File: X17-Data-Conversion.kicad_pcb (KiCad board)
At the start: 2 copper layers, 41.5 x 30.7 mm, 28 parts, among them J1 Conn_01x05, J4 Conn_01x12_Pin, U2 STM32F091CCTx, U3 MAX485E, U4 MAX7375AXR805+T, U5 AZ1117IH-3.3TRG1

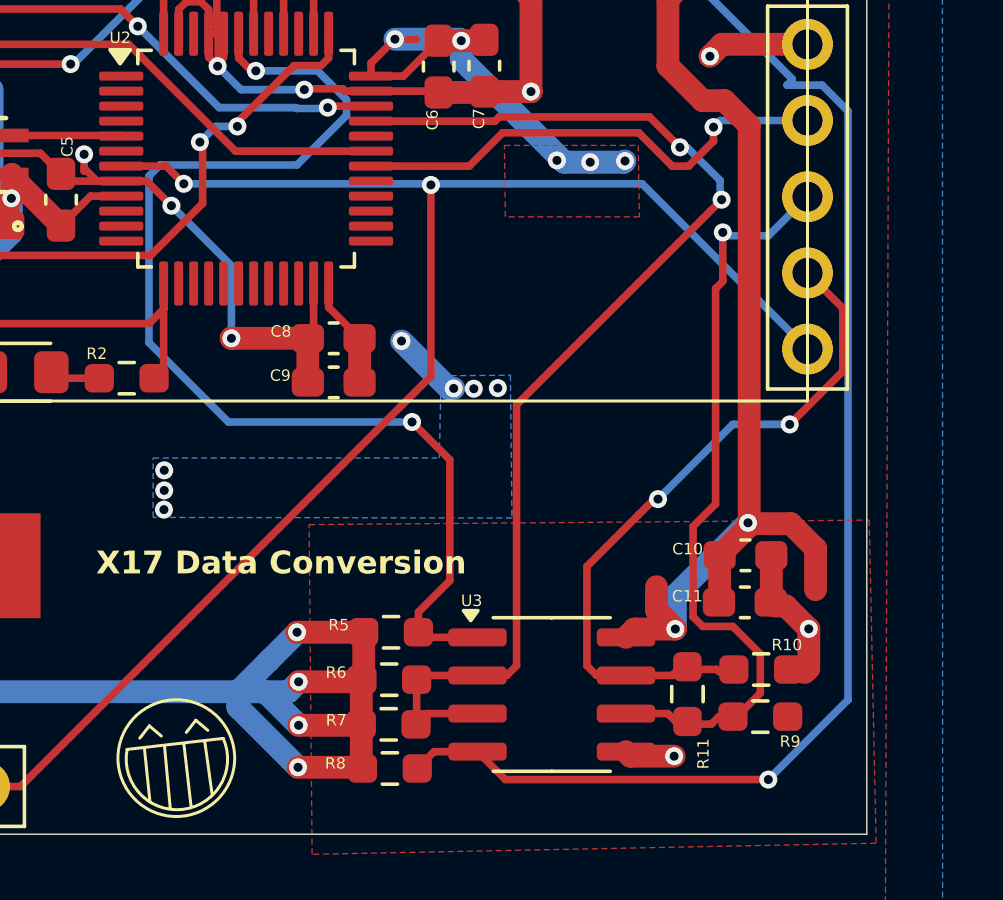
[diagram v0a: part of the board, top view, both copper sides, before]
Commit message: daniel lookie
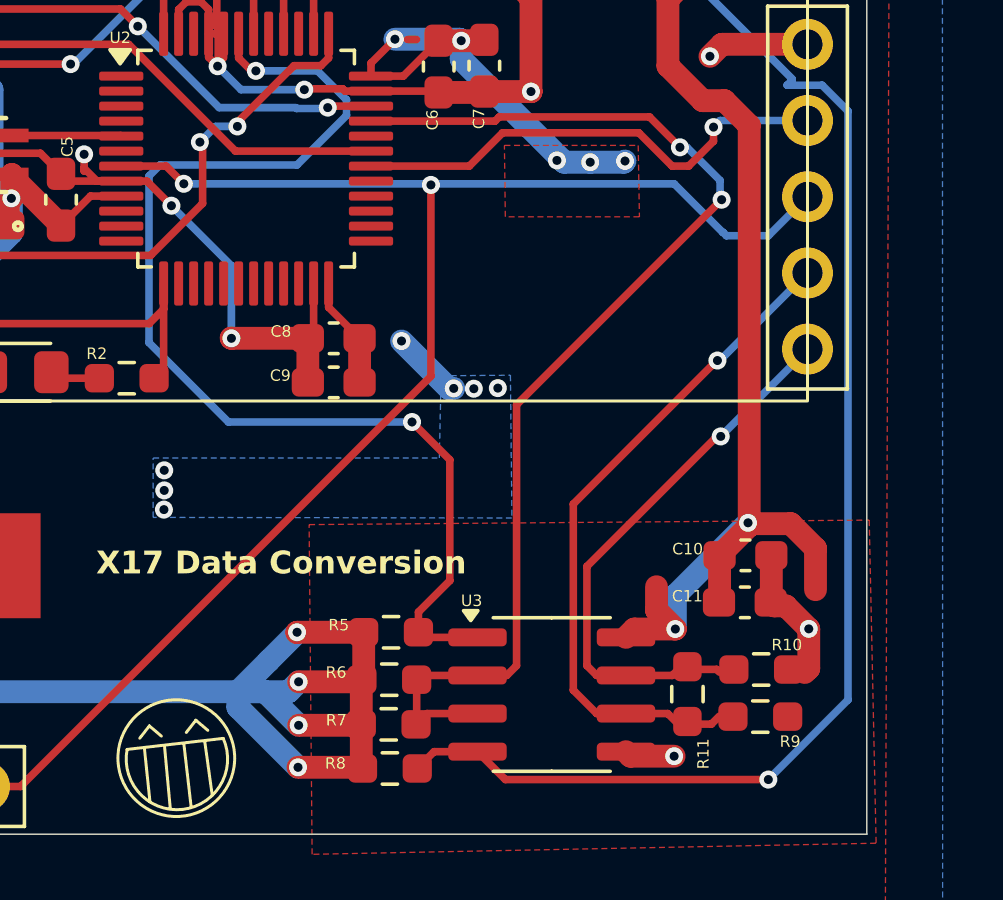
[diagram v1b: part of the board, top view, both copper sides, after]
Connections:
- J4 pad 10: A+ -> NRST_PSB
- J4 pad 11: A- -> A+
- J4 pad 12: NRST_PSB -> A-
- J4 pad 3: SWDIO -> unconnected-(J4-Pin_3-Pad3)
- J4 pad 4: SWCLK -> unconnected-(J4-Pin_4-Pad4)
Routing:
- net A-: track 23.4 -> 18.7 mm, vias 2 -> 1
- net A+: track 25.3 -> 22.8 mm
- net NRST_PSB: track 52.3 -> 51.3 mm
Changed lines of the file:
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@@
 	(net 44 "Net-(U2-PF0)")
 	(net 45 "unconnected-(U2-PF1-Pad6)")
+	(net 46 "unconnected-(J4-Pin_3-Pad3)")
+	(net 47 "unconnected-(J4-Pin_4-Pad4)")
 	(footprint "Capacitor_SMD:C_0603_1608Metric_Pad1.08x0.95mm_HandSolder"
 		(layer "F.Cu")
@@
 			(layers "*.Cu" "*.Mask")
 			(remove_unused_layers no)
-			(net 5 "SWDIO")
+			(net 46 "unconnected-(J4-Pin_3-Pad3)")
 			(pinfunction "Pin_3")
-			(pintype "passive")
+			(pintype "passive+no_connect")
 		)
 		(pad "4" thru_hole oval
@@
 			(layers "*.Cu" "*.Mask")
 			(remove_unused_layers no)
-			(net 4 "SWCLK")
+			(net 47 "unconnected-(J4-Pin_4-Pad4)")
 			(pinfunction "Pin_4")
-			(pintype "passive")
+			(pintype "passive+no_connect")
 		)
 		(pad "5" thru_hole oval
@@
 			(layers "*.Cu" "*.Mask")
 			(remove_unused_layers no)
-			(net 11 "A+")
+			(net 1 "NRST_PSB")
 			(pinfunction "Pin_10")
 			(pintype "passive")
@@
 			(layers "*.Cu" "*.Mask")
 			(remove_unused_layers no)
-			(net 12 "A-")
+			(net 11 "A+")
 			(pinfunction "Pin_11")
 			(pintype "passive")
@@
 			(layers "*.Cu" "*.Mask")
 			(remove_unused_layers no)
-			(net 1 "NRST_PSB")
+			(net 12 "A-")
 			(pinfunction "Pin_12")
 			(pintype "passive")
@@
 		)
 		(property "Value" "MAX7375AXR805+T"
-			(at 1.21 -2.07 90)
+			(at 0 0 90)
 			(unlocked yes)
 			(layer "F.Fab")
 			(effects
 				(font
-					(size 0.381 0.381)
-					(thickness 0.03175)
+					(size 1 1)
+					(thickness 0.15)
 				)
 			)
@@
 	)
 	(segment
-		(start 159.483 75.03)
-		(end 174.7625 75.03)
+		(start 177.449 76.65)
+		(end 177.46 76.65)
+		(width 0.254)
+		(layer "B.Cu")
+		(net 1)
+	)
+	(segment
+		(start 177.46 76.65)
+		(end 177.570224 76.760224)
+		(width 0.254)
+		(layer "B.Cu")
+		(net 1)
+	)
+	(segment
+		(start 177.570224 76.760224)
+		(end 178.972276 76.760224)
 		(width 0.254)
 		(layer "B.Cu")
@@
 	(segment
 		(start 159.483 75.03)
-		(end 159.473 75.04)
+		(end 175.829 75.03)
 		(width 0.254)
 		(layer "B.Cu")
@@
 	)
 	(segment
-		(start 174.7625 75.03)
-		(end 180.2725 80.54)
+		(start 175.829 75.03)
+		(end 177.449 76.65)
+		(width 0.254)
+		(layer "B.Cu")
+		(net 1)
+	)
+	(segment
+		(start 178.972276 76.760224)
+		(end 180.2725 75.46)
+		(width 0.254)
+		(layer "B.Cu")
+		(net 1)
+	)
+	(segment
+		(start 159.483 75.03)
+		(end 159.473 75.04)
 		(width 0.254)
 		(layer "B.Cu")
@@
 	)
 	(segment
-		(start 177.784014 89.784014)
-		(end 178.7 90.7)
-		(width 0.254)
-		(layer "F.Cu")
-		(net 11)
-	)
-	(segment
 		(start 175.6145 92.688264)
 		(end 175.967 93.040764)
@@
 	)
 	(segment
-		(start 178.7 90.7)
-		(end 178.7 92.01)
-		(width 0.254)
-		(layer "F.Cu")
-		(net 11)
-	)
-	(segment
-		(start 176.781596 89.784014)
-		(end 177.784014 89.784014)
+		(start 173.247001 92.688264)
+		(end 174.222 92.688264)
 		(width 0.254)
 		(layer "F.Cu")
@@
 	)
 	(segment
-		(start 177.449 76.65)
-		(end 177.449 78.2835)
+		(start 177.25 80.92)
+		(end 172.466 85.704)
 		(width 0.254)
 		(layer "F.Cu")
@@
 	)
 	(segment
-		(start 177.449 78.2835)
-		(end 177.21 78.5225)
-		(width 0.254)
-		(layer "F.Cu")
-		(net 11)
-	)
-	(segment
-		(start 176.4575 86.45261)
-		(end 176.4575 89.459918)
+		(start 172.466 91.907263)
+		(end 173.247001 92.688264)
 		(width 0.254)
 		(layer "F.Cu")
@@
 	)
 	(segment
-		(start 177.21 85.70011)
-		(end 176.4575 86.45261)
+		(start 177.27 80.92)
+		(end 177.25 80.92)
 		(width 0.254)
 		(layer "F.Cu")
@@
 	)
 	(segment
-		(start 177.21 78.5225)
-		(end 177.21 85.70011)
-		(width 0.254)
-		(layer "F.Cu")
-		(net 11)
-	)
-	(segment
-		(start 178.7 92.01)
-		(end 177.92 92.79)
-		(width 0.254)
-		(layer "F.Cu")
-		(net 11)
-	)
-	(segment
-		(start 176.4575 89.459918)
-		(end 176.781596 89.784014)
+		(start 172.466 85.704)
+		(end 172.466 91.907263)
 		(width 0.254)
 		(layer "F.Cu")
@@
 	)
 	(via
-		(at 177.449 76.65)
+		(at 177.27 80.92)
 		(size 0.6)
 		(drill 0.3)
@@
 	)
 	(segment
-		(start 178.972276 76.760224)
-		(end 177.570224 76.760224)
-		(width 0.254)
-		(layer "B.Cu")
-		(net 11)
-	)
-	(segment
-		(start 177.46 76.65)
-		(end 177.449 76.65)
-		(width 0.254)
-		(layer "B.Cu")
-		(net 11)
-	)
-	(segment
-		(start 180.2725 75.46)
-		(end 178.972276 76.760224)
+		(start 177.3525 80.92)
+		(end 180.2725 78)
 		(width 0.254)
 		(layer "B.Cu")
@@
 	)
 	(segment
-		(start 177.570224 76.760224)
-		(end 177.46 76.65)
+		(start 177.27 80.92)
+		(end 177.3525 80.92)
 		(width 0.254)
 		(layer "B.Cu")
@@
 	)
 	(segment
-		(start 175.163 85.54)
-		(end 174.643 86.06)
-		(width 0.254)
-		(layer "F.Cu")
-		(net 12)
-	)
-	(segment
-		(start 174.643 86.06)
-		(end 172.92 87.783)
+		(start 173.247001 91.418264)
+		(end 174.222 91.418264)
 		(width 0.254)
 		(layer "F.Cu")
@@
 	)
 	(segment
-		(start 175.29 85.54)
-		(end 175.163 85.54)
+		(start 172.92 87.783)
+		(end 172.92 91.091263)
 		(width 0.254)
 		(layer "F.Cu")
@@
 	)
 	(segment
-		(start 181.4495 79.177)
-		(end 181.4495 81.2805)
-		(width 0.254)
-		(layer "F.Cu")
-		(net 12)
-	)
-	(segment
 		(start 175.967 91.215764)
 		(end 177.247 91.215764)
@@
 	)
 	(segment
-		(start 180.2725 78)
-		(end 181.4495 79.177)
+		(start 177.253 83.45)
+		(end 172.92 87.783)
 		(width 0.254)
 		(layer "F.Cu")
@@
 	)
 	(segment
-		(start 173.247001 91.418264)
-		(end 174.222 91.418264)
+		(start 177.38 83.45)
+		(end 177.253 83.45)
 		(width 0.254)
 		(layer "F.Cu")
@@
 	)
 	(segment
-		(start 181.4495 81.2805)
-		(end 179.68 83.05)
-		(width 0.254)
-		(layer "F.Cu")
-		(net 12)
-	)
-	(segment
-		(start 172.92 87.783)
-		(end 172.92 91.091263)
-		(width 0.254)
-		(layer "F.Cu")
-		(net 12)
-	)
-	(segment
 		(start 173.838264 91.418264)
 		(end 174.222 91.418264)
@@
 	)
 	(via
-		(at 179.68 83.05)
-		(size 0.6)
-		(drill 0.3)
-		(layers "F.Cu" "B.Cu")
-		(net 12)
-	)
-	(via
-		(at 175.29 85.54)
+		(at 177.38 83.45)
 		(size 0.6)
 		(drill 0.3)
@@
 	)
 	(segment
-		(start 179.68 83.05)
-		(end 177.78 83.05)
+		(start 180.2725 80.5575)
+		(end 180.2725 80.54)
 		(width 0.254)
 		(layer "B.Cu")
@@
 	)
 	(segment
-		(start 177.78 83.05)
-		(end 175.29 85.54)
+		(start 177.38 83.45)
+		(end 180.2725 80.5575)
 		(width 0.254)
 		(layer "B.Cu")
